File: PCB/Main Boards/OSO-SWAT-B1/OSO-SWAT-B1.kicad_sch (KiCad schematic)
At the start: 35 parts, among them J1 OSO_SWD, U1 ATSAML22J18A-MUT, U2 MIC5365-3.3YC5-TR, X1 Crystal

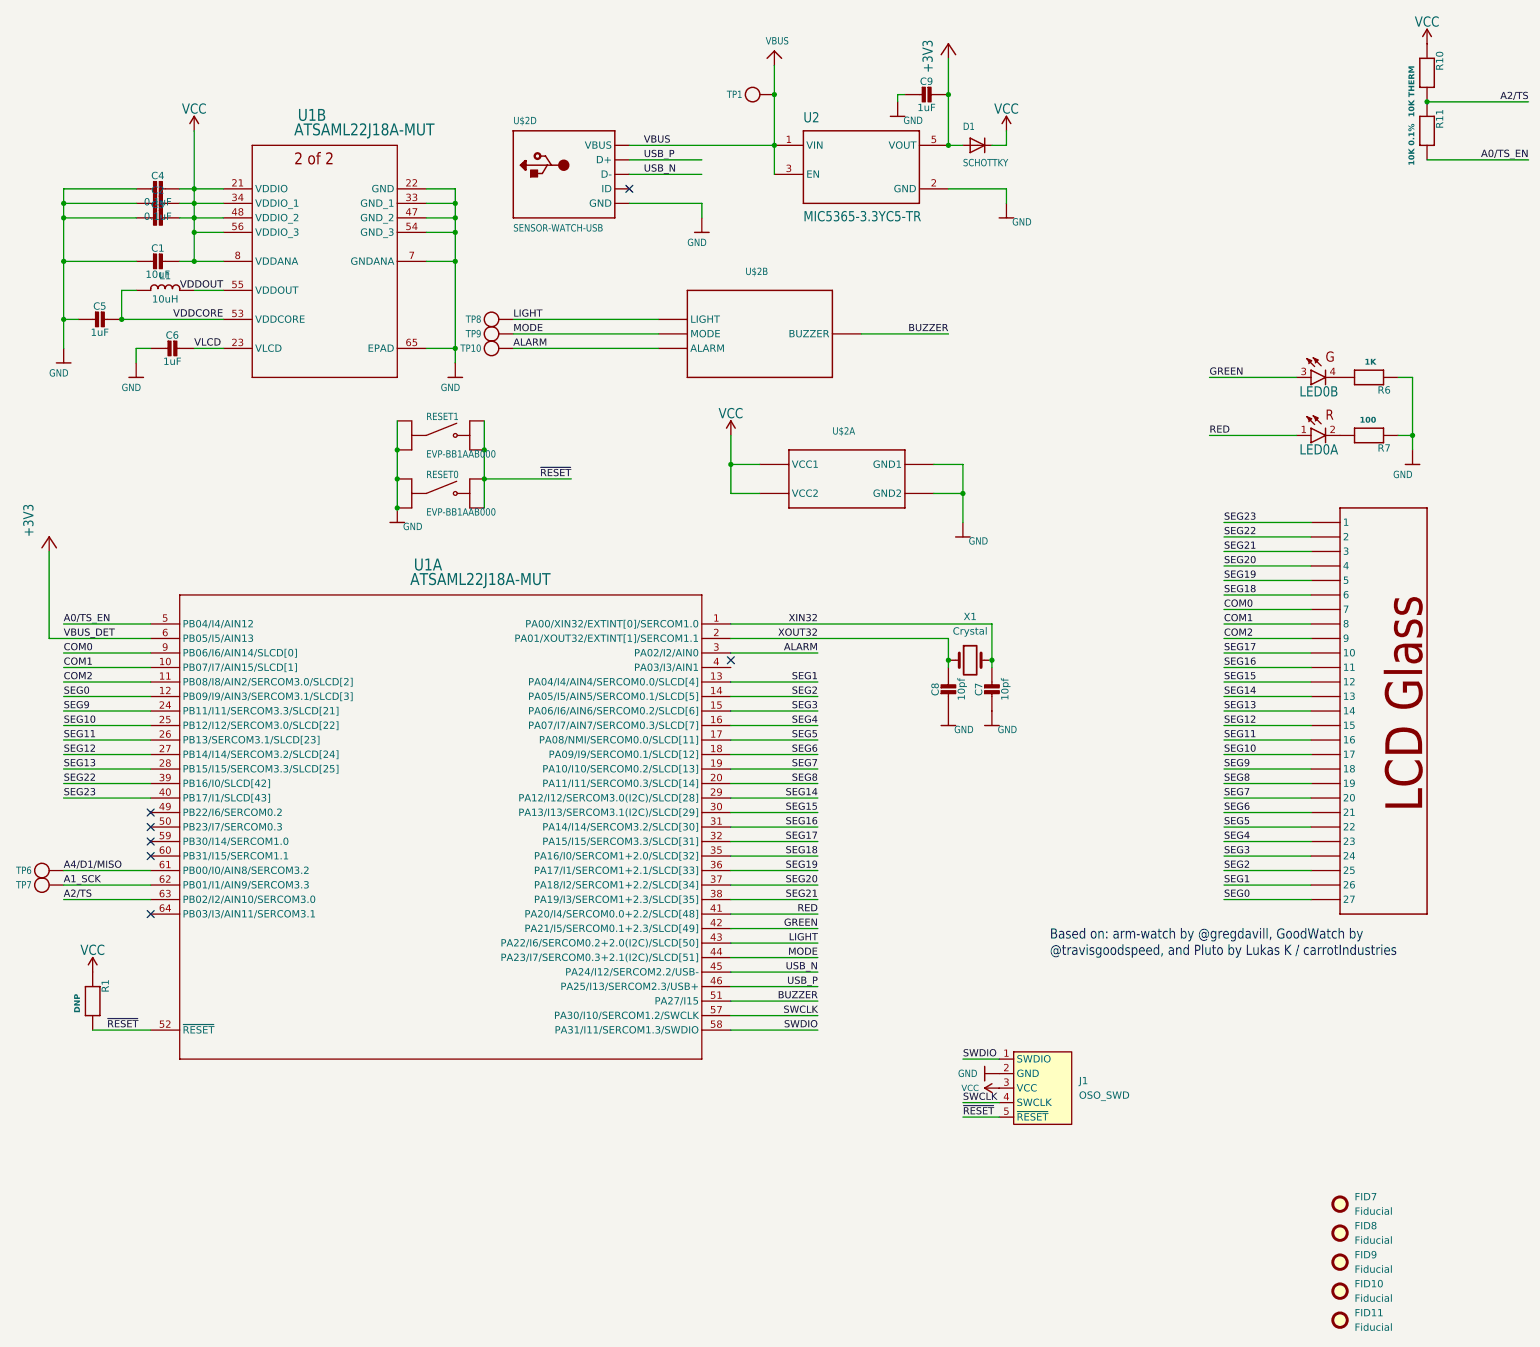
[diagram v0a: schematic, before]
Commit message: WIP buzzer protection
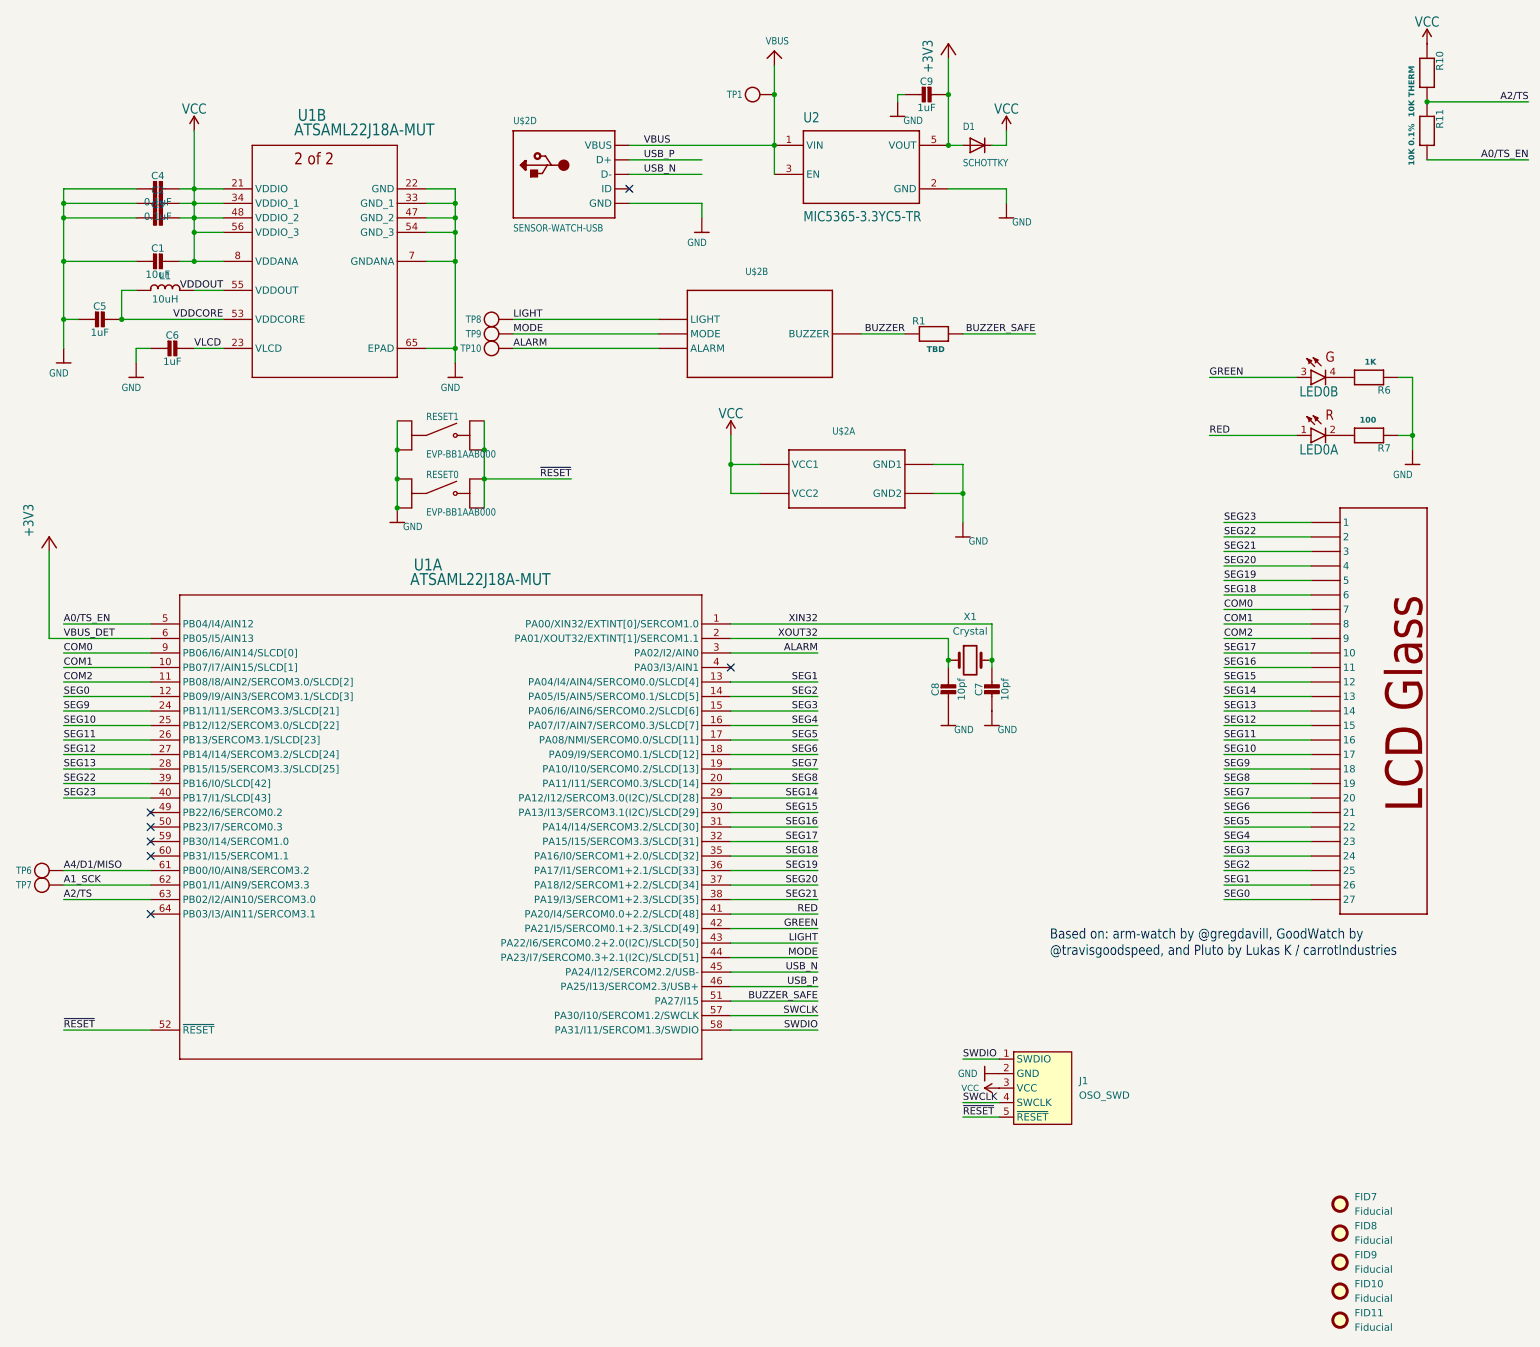
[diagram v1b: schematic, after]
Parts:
- R1: value DNP -> TBD
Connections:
- net BUZZER: now also R1.1; no longer U1.51 (PA27/I15)
- net VCC: no longer R1.1
- net ~{RESET}: no longer R1.2
- new net BUZZER_SAFE: R1.2, U1.51 (PA27/I15)
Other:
- moved on the sheet: R1
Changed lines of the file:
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@@
 (kicad_sch (version 20211123) (generator eeschema)
-  (paper "User" 300.507 242.062)
+  (paper "USLetter")
+  (title_block
+    (date "2023-01-23")
+    (rev "02")
+  )
   (junction (at 88.9 93.98) (diameter 0) (color 0 0 0 0)
   )
@@
   (no_connect (at 45.72 165.1))
   (no_connect (at 129.54 38.1))
-  (no_connect (at 147.32 120.65))
+  (no_connect (at 147.32 121.92))
   (no_connect (at 45.72 152.4))
   (no_connect (at 45.72 154.94))
@@
     (stroke (width 0) (type default) (color 0 0 0 0))
   )
+  (wire (pts (xy 30.48 185.42) (xy 45.72 185.42))
+    (stroke (width 0) (type default) (color 0 0 0 0))
+  )
   (wire (pts (xy 233.68 124.46) (xy 248.92 124.46))
     (stroke (width 0) (type default) (color 0 0 0 0))
@@
     (stroke (width 0) (type default) (color 0 0 0 0))
   )
+  (wire (pts (xy 200.66 63.5) (xy 187.96 63.5))
+    (stroke (width 0) (type default) (color 0 0 0 0))
+  )
   (wire (pts (xy 269.24 22.86) (xy 287.02 22.86))
     (stroke (width 0) (type default) (color 0 0 0 0))
@@
     (stroke (width 0) (type default) (color 0 0 0 0))
   )
-  (wire (pts (xy 35.56 185.42) (xy 45.72 185.42))
-    (stroke (width 0) (type default) (color 0 0 0 0))
-  )
   (wire (pts (xy 30.48 139.7) (xy 45.72 139.7))
     (stroke (width 0) (type default) (color 0 0 0 0))
   )
-  (wire (pts (xy 185.42 63.5) (xy 170.18 63.5))
+  (wire (pts (xy 177.8 63.5) (xy 170.18 63.5))
     (stroke (width 0) (type default) (color 0 0 0 0))
   )
@@
     (effects (font (size 1.2446 1.2446)) (justify right bottom))
   )
-  (label "~{RESET}" (at 38.1 185.42 0)
+  (label "~{RESET}" (at 30.48 185.42 0)
     (effects (font (size 1.2446 1.2446)) (justify left bottom))
   )
@@
     (effects (font (size 1.2446 1.2446)) (justify left bottom))
   )
-  (label "BUZZER" (at 162.56 180.34 180)
+  (label "BUZZER_SAFE" (at 162.56 180.34 180)
+    (effects (font (size 1.2446 1.2446)) (justify right bottom))
+  )
+  (label "BUZZER_SAFE" (at 200.66 63.5 180)
     (effects (font (size 1.2446 1.2446)) (justify right bottom))
   )
@@
     (effects (font (size 1.2446 1.2446)) (justify right bottom))
   )
-  (label "BUZZER" (at 185.42 63.5 180)
+  (label "BUZZER" (at 177.8 63.5 180)
     (effects (font (size 1.2446 1.2446)) (justify right bottom))
   )
@@
     (pin "2")
   )
-  (symbol (lib_id "OSO-SWAT-A1-05-eagle-import:RESISTOR_0603MP") (at 35.56 180.34 270) (unit 1)
-    (in_bom yes) (on_board yes)
-    (property "Reference" "R1" (id 0) (at 37.0586 176.53 0)
+  (symbol (lib_id "OSO-SWAT-A1-05-eagle-import:RESISTOR_0603MP") (at 182.88 63.5 0) (unit 1)
+    (in_bom yes) (on_board yes)
+    (property "Reference" "R1" (id 0) (at 179.07 62.0014 0)
       (effects (font (size 1.27 1.27)) (justify left bottom))
     )
-    (property "Value" "DNP" (id 1) (at 32.258 179.07 0)
+    (property "Value" "TBD" (id 1) (at 181.61 66.802 0)
       (effects (font (size 1.016 1.016) bold) (justify left bottom))
     )
-    (property "Footprint" "OSO-SWAT-A1-05:_0603MP" (id 2) (at 35.56 180.34 0)
-      (effects (font (size 1.27 1.27)) hide)
-    )
-    (property "Datasheet" "" (id 3) (at 35.56 180.34 0)
+    (property "Footprint" "OSO-SWAT-A1-05:_0603MP" (id 2) (at 182.88 63.5 0)
+      (effects (font (size 1.27 1.27)) hide)
+    )
+    (property "Datasheet" "" (id 3) (at 182.88 63.5 0)
       (effects (font (size 1.27 1.27)) hide)
     )
@@
     (pin "1")
   )
-  (symbol (lib_id "OSO-SWAT-A1-05-eagle-import:VCC") (at 35.56 175.26 0) (unit 1)
-    (in_bom yes) (on_board yes)
-    (property "Reference" "#SUPPLY05" (id 0) (at 35.56 175.26 0)
-      (effects (font (size 1.27 1.27)) hide)
-    )
-    (property "Value" "VCC" (id 1) (at 35.56 172.466 0)
-      (effects (font (size 1.778 1.5113)) (justify bottom))
-    )
-    (property "Footprint" "OSO-SWAT-A1-05:" (id 2) (at 35.56 175.26 0)
-      (effects (font (size 1.27 1.27)) hide)
-    )
-    (property "Datasheet" "" (id 3) (at 35.56 175.26 0)
-      (effects (font (size 1.27 1.27)) hide)
-    )
-    (pin "1")
-  )
   (symbol (lib_id "OSO-SWAT-A1-05-eagle-import:QBLP655-RIG") (at 248.92 71.12 0) (unit 2)
     (in_bom yes) (on_board yes)
@@
       (reference "#SUPPLY02") (unit 1) (value "VCC") (footprint "OSO-SWAT-A1-05:")
     )
-    (path "/5d1f1286-1612-4034-9350-9e814aa8acc2"
-      (reference "#SUPPLY05") (unit 1) (value "VCC") (footprint "OSO-SWAT-A1-05:")
-    )
     (path "/ba33d7b0-79fd-4ba9-85f0-0eae394abc9f"
       (reference "#SUPPLY08") (unit 1) (value "VCC") (footprint "OSO-SWAT-A1-05:")
@@
     )
     (path "/2a410890-4cb7-4214-ae06-c49d77d71777"
-      (reference "R1") (unit 1) (value "DNP") (footprint "OSO-SWAT-A1-05:_0603MP")
+      (reference "R1") (unit 1) (value "TBD") (footprint "OSO-SWAT-A1-05:_0603MP")
     )
     (path "/1050a4b5-88c4-4068-ab0b-d9b191a3a97f"
